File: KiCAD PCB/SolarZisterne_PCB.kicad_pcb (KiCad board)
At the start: 2 copper layers, 99.1 x 74.3 mm, 29 parts, among them J1 Erzeugung, J10 GS2, J11 GS2, J12 GS2, J13 GS2, J14 Buck-Conv D24V5F3, J2 Verbrauch, J3 Solar, J4 Akku, J5 Ultraschall Sensor, J6 Externer Temperatur Sensor, J7 Interner Temperatur Sensor, J8 Erweiterung, J9 GS2, U2 MCP73871, U3 WeMos_mini, U4 MCP23008

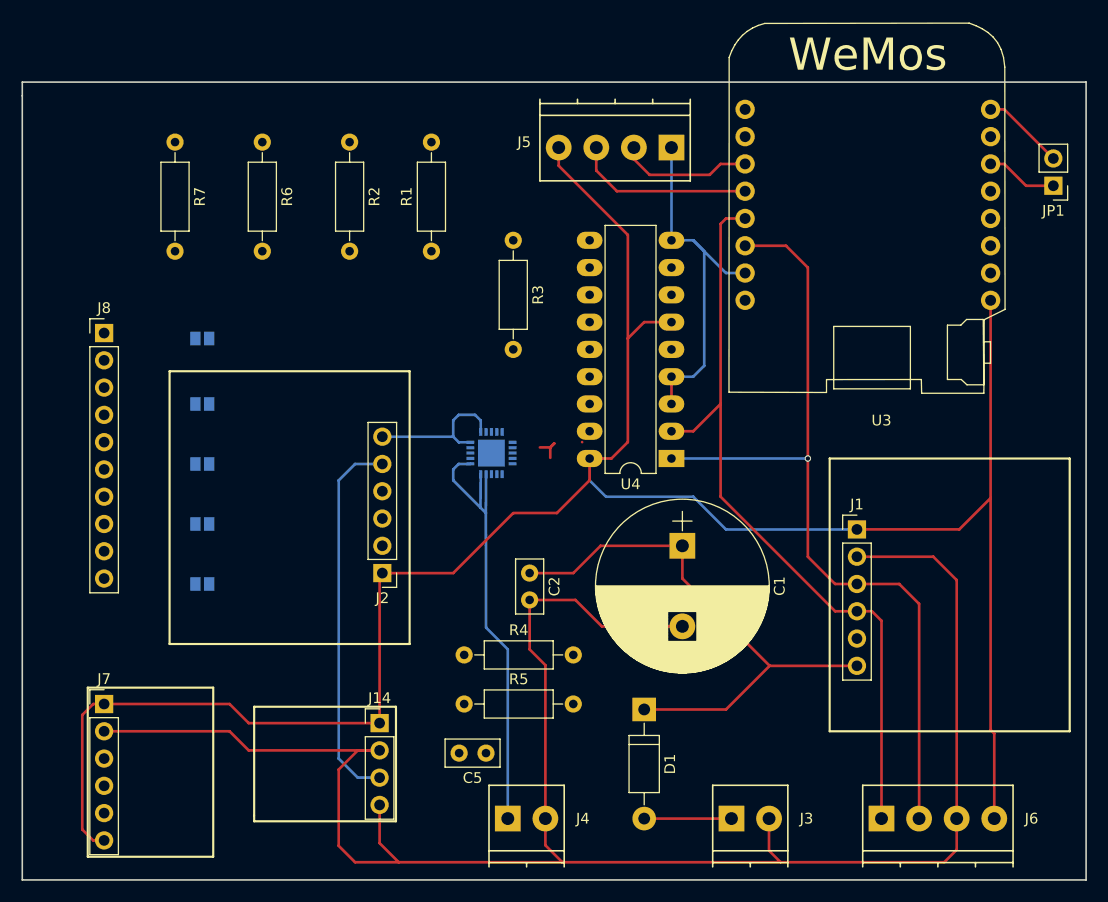
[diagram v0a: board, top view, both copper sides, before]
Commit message: fast aller Leiterbahnen
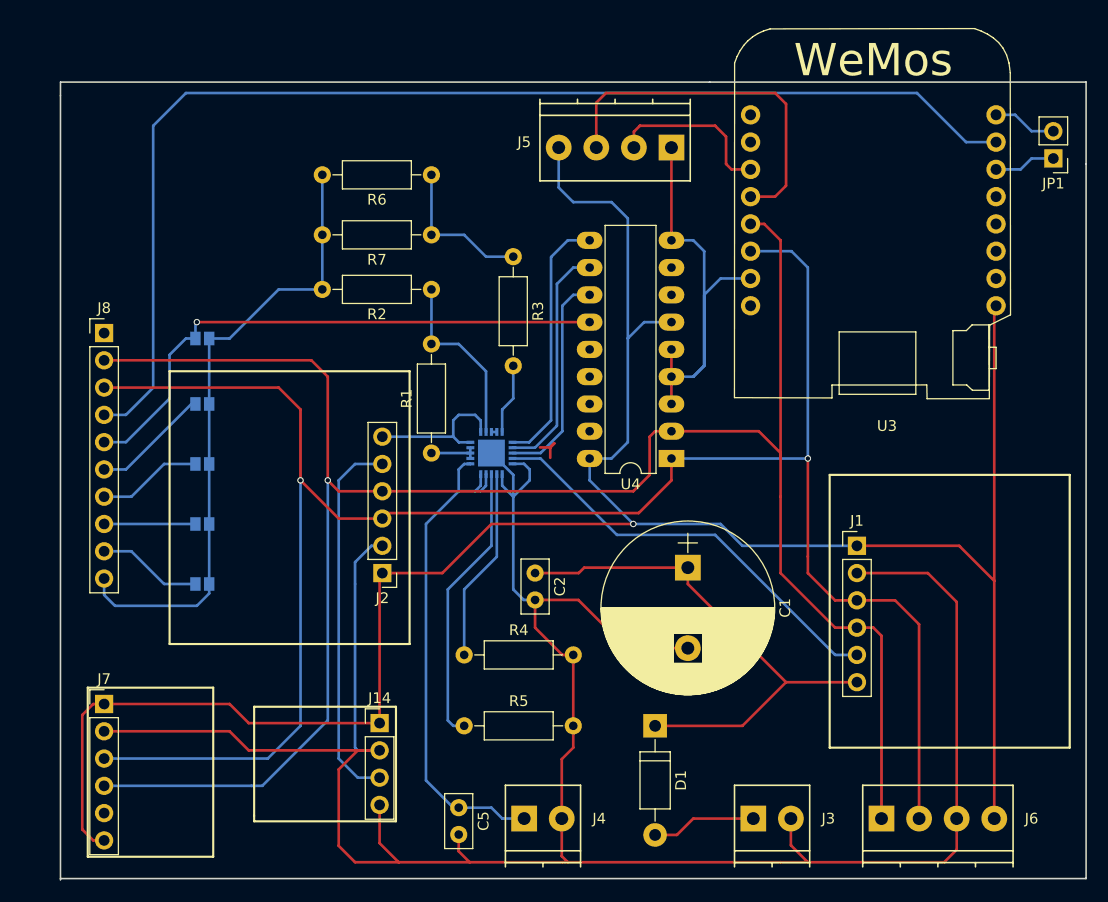
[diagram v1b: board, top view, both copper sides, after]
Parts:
- U3: value WeMos_mini -> WeMos_Mini
- moved R7 25.4 mm to (157.5, 54.9), turned to 180 degrees
- moved R1 18.8 mm to (157.5, 75.2)
- moved R6 16.0 mm to (157.5, 49.3), turned to 180 degrees
- moved R2 15.7 mm to (157.5, 59.9), turned to 180 degrees
- moved C5 5.68 mm to (160.0, 108.2), turned to 270 degrees
- moved JP1 2.54 mm to (215.4, 47.8)
- moved C1 2.09 mm to (181.4, 85.9)
- moved J3 2.03 mm to (187.5, 109.2)
- moved R5 2.03 mm to (160.5, 100.6)
- moved D1 1.83 mm to (178.3, 100.6)
- moved J4 1.52 mm to (166.1, 109.2)
- moved R3 1.52 mm to (165.1, 56.9)
- moved J1 1.52 mm to (197.1, 83.8)
- moved U3 0.72 mm to (198.6, 53.8)
- moved C2 0.51 mm to (167.1, 86.4)
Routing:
- net GND: track 218.5 -> 336.1 mm
- net /SDA: track 71.7 -> 188.4 mm, vias 0 -> 1
- net /Analog1: track 0.00 -> 111.7 mm
- net /SCL: track 78.5 -> 185.2 mm, vias 1 -> 2
- net /GPB3: track 0.00 -> 53.0 mm, vias 0 -> 1
- net VCC: track 0.00 -> 44.8 mm
- net Net-(R5-Pad1): track 0.00 -> 26.9 mm
- net /PG: track 1.02 -> 24.9 mm
- net /STAT2: track 0.00 -> 21.9 mm
- net /STAT1: track 0.00 -> 20.1 mm
- net Net-(R4-Pad1): track 0.00 -> 18.1 mm
- net /Trig: track 16.8 -> 34.0 mm
- net Net-(R1-Pad2): track 0.00 -> 16.9 mm
- net Net-(R3-Pad1): track 0.00 -> 14.0 mm
- net /GPB4: track 0.00 -> 11.0 mm
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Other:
- board size 99.1 x 74.3 mm -> 95.5 x 74.3 mm
